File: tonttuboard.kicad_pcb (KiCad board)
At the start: 4 copper layers, 72.5 x 22.5 mm, 45 parts, among them U3 ICM-40609-D, U4 BMP388, U5 W25Q256JVFIQT, U6 MMC5983MA, U9 Teensy 4.0

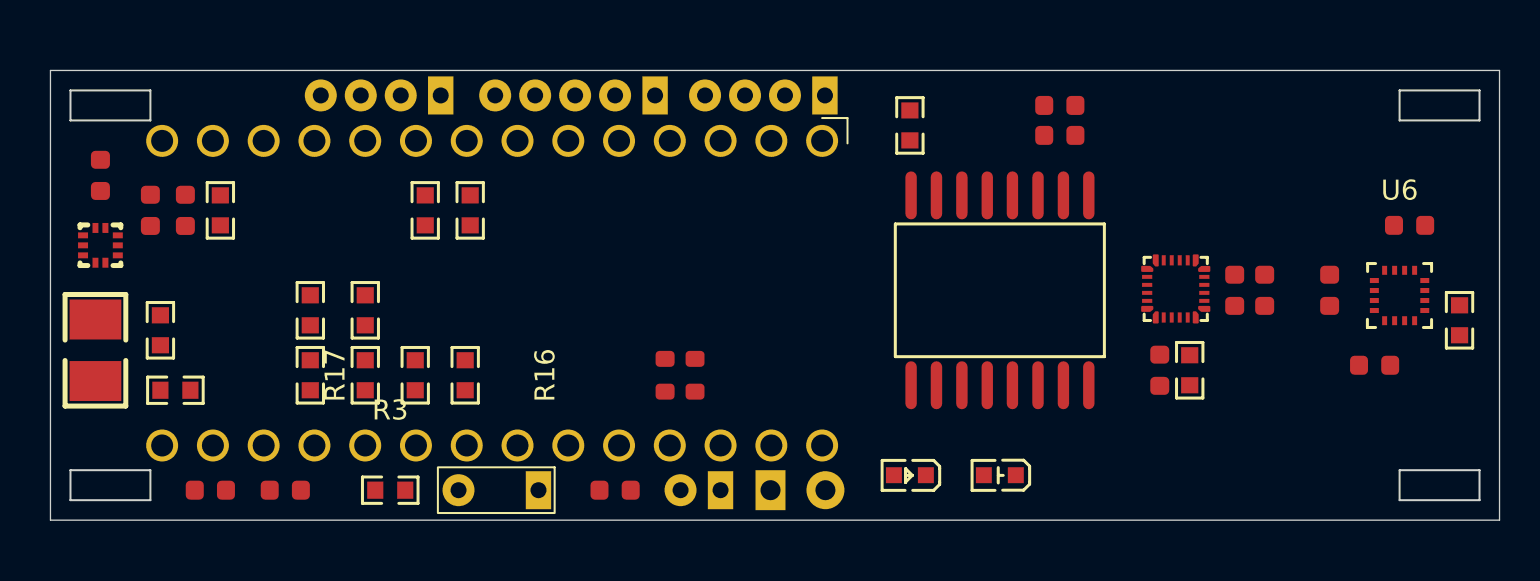
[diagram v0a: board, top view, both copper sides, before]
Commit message: Routed signals
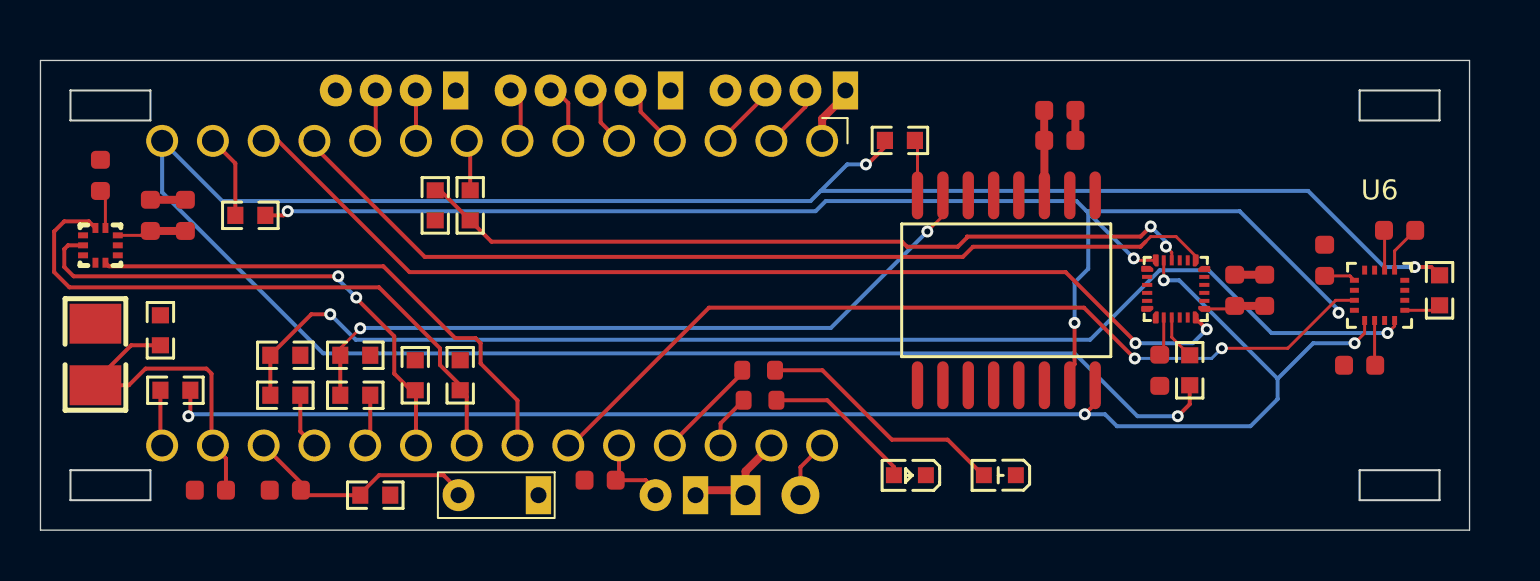
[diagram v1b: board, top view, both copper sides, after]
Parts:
- moved R15 4.69 mm to (110.4, 90.0), turned to 0 degrees
- moved R19 3.48 mm to (110.5, 91.5), turned to 0 degrees
- moved R20 2.57 mm to (86.8, 89.2), turned to 0 degrees
- moved R21 2.30 mm to (90.2, 89.2), turned to 0 degrees
- moved R6 1.80 mm to (144.5, 86.0), turned to 90 degrees
- moved R12 1.60 mm to (86.8, 91.2), turned to 180 degrees
- moved C8 1.52 mm to (138.8, 84.5), turned to -90 degrees
- moved R13 1.52 mm to (85.0, 82.2), turned to 180 degrees
- moved U2 1.27 mm to (112.3, 96.2)
- moved U7 1.27 mm to (104.8, 96.2)
- moved R11 1.12 mm to (90.2, 91.2), turned to 0 degrees
- moved U10 1.06 mm to (119.8, 76.0)
- moved U6 1.00 mm to (141.5, 86.2)
- moved C14 0.90 mm to (102.5, 95.5)
- moved R5 0.90 mm to (117.5, 78.5), turned to 180 degrees
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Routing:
- net MISO: track 0.00 -> 131.4 mm, vias 0 -> 3
- net CLOCK: track 0.00 -> 74.0 mm, vias 0 -> 4
- net MOSI: track 0.00 -> 70.9 mm, vias 0 -> 4
- net CS_MAG: track 0.00 -> 62.8 mm, vias 0 -> 2
- net IMU_INT1: track 0.00 -> 52.5 mm, vias 0 -> 2
- net IMU_INT2: track 0.00 -> 47.8 mm
- net MAG_INT: track 0.00 -> 44.7 mm, vias 0 -> 2
- net CS_IMU: track 0.00 -> 39.5 mm, vias 0 -> 2
- net CS_FLASH: track 0.00 -> 36.3 mm, vias 0 -> 2
- net SCL: track 0.00 -> 30.9 mm
- net BARO_INT: track 0.00 -> 26.3 mm
- net SDA: track 0.00 -> 26.2 mm, vias 0 -> 2
- net +3.3V: track 0.00 -> 21.5 mm
- net LDR_READ: track 0.00 -> 16.4 mm
- net GND: track 0.00 -> 15.3 mm
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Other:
- board size 72.5 x 22.5 mm -> 71.5 x 23.5 mm

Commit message: Added gnd vias and decorated
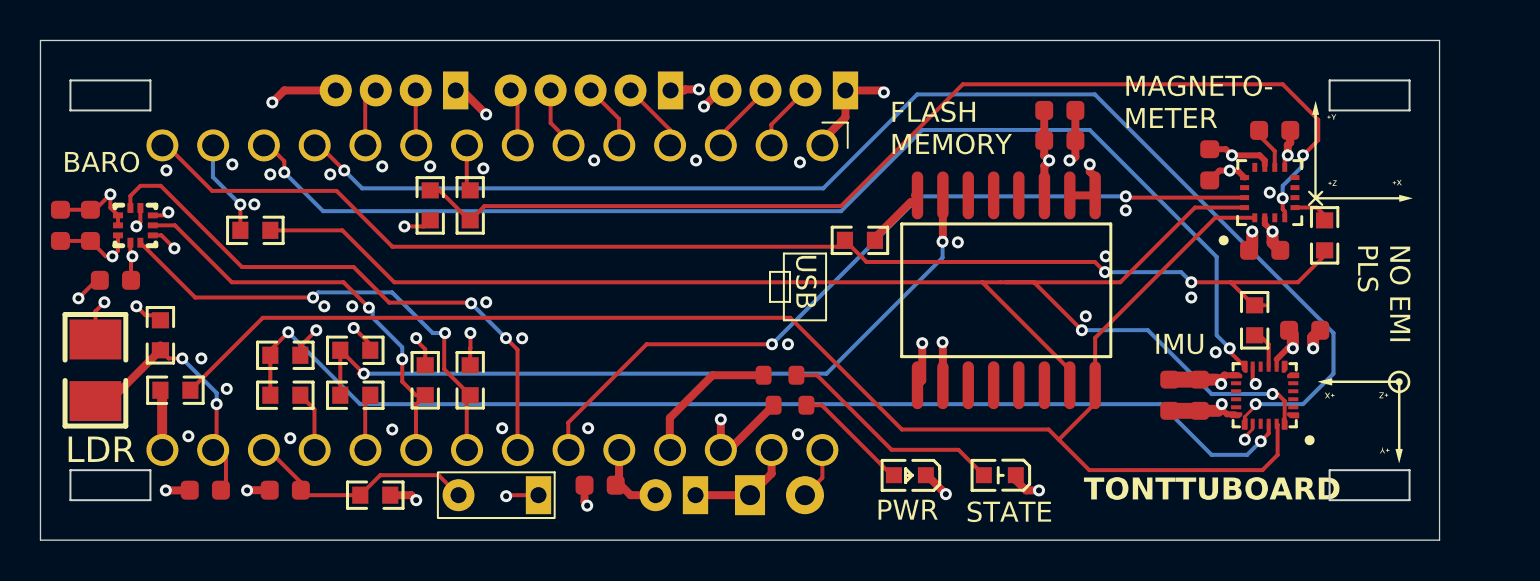
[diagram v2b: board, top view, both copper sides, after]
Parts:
- added G***: LOGO, Graphics:mag_orientation_6x5,5, F.Cu at (140.5, 79.2)
- added G***: LOGO, Graphics:imu_orientation_6,5x5, F.Cu at (140.8, 92.2)
- added G***: LOGO, Graphics:ekotomtarna_nino_logo_22x22_positive, B.Cu at (127.2, 85.4)
- moved C5 8.00 mm to (136.2, 78.0)
- moved U6 7.52 mm to (136.0, 81.1)
- moved C15 7.52 mm to (137.8, 88.0), turned to 180 degrees
- moved C8 7.48 mm to (133.0, 79.7)
- moved C11 7.46 mm to (135.8, 84.0)
- moved C2 7.08 mm to (131.0, 91.2), turned to -90 degrees
- moved U3 6.94 mm to (135.8, 91.2), turned to 180 degrees
- moved R6 6.37 mm to (138.8, 83.2), turned to -90 degrees
- moved C16 5.53 mm to (132.5, 91.2), turned to -90 degrees
- moved R5 5.39 mm to (115.5, 83.5)
- moved C4 5.30 mm to (78.2, 85.5), turned to 0 degrees
- moved C1 4.78 mm to (77.0, 82.8)
- moved C3 4.53 mm to (75.5, 82.8)
- moved R1 4.10 mm to (135.2, 87.5), turned to 90 degrees
- moved U4 2.02 mm to (79.2, 82.8), turned to 180 degrees
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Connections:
- R10 pad 1: CS_IMU -> CS_MAG
- R12 pad 2: CS_MAG -> CS_IMU
- R20 pad 1: CS_MAG -> CS_IMU
- R9 pad 1: CS_IMU -> CS_MAG
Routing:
- net MISO: track 131.4 -> 65.0 mm, vias 3 -> 2
- net GND: track 15.3 -> 50.0 mm, vias 0 -> 54
- net +3.3V: track 21.5 -> 48.6 mm, vias 0 -> 20
- net IMU_INT2: track 47.8 -> 66.6 mm, vias 0 -> 2
- net CS_IMU: track 39.5 -> 56.0 mm
- net CS_MAG: track 62.8 -> 54.5 mm
- net IMU_INT1: track 52.5 -> 59.9 mm
- net SCL: track 30.9 -> 23.6 mm, vias 0 -> 2
- net SDA: track 26.2 -> 21.1 mm
- net MOSI: track 70.9 -> 75.9 mm, vias 4 -> 2
- net MAG_INT: track 44.7 -> 39.7 mm
- net CLOCK: track 74.0 -> 78.2 mm, vias 4 -> 0
- net CS_FLASH: track 36.3 -> 38.7 mm
- net BARO_INT: track 26.3 -> 28.4 mm, vias 0 -> 2
- net Net-(LED1-A): track 7.68 -> 6.02 mm
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- added copper zone on In2.Cu, net +3.3V
- added copper zone on In1.Cu, net GND
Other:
- board size 71.5 x 23.5 mm -> 70 x 25 mm
- board text added: "3V"
- board text added: "5V"
- board text added: "BARO"
- board text added: "BAT_READ"
- board text added: "EKOTOMTARNA"
- board text added: "FLASH MEMORY"
- board text added: "IMU"
- board text added: "M1"
- board text added: "M2"
- board text added: "M3"
- board text added: "M4"
- board text added: "MAGNETO- METER"
- board text added: "NO EMI PLS"
- board text added: "PWR"
- board text added: "RX"
- board text added: "STATE"
- board text added: "THERM."
- board text added: "TONTTUBOARD"
- board text added: "TX"
- board text added: "USB"
- board text added: "{dblquote}DESIGNED{dblquote} BY OSKAR HUOTARI"
